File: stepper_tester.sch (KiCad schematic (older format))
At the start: 19 parts, among them J1 Conn_01x08, J2 Conn_01x08, J3 Conn_01x04, J4 Conn_01x03, J5 Conn_01x01, J6 Conn_01x01, J7 Conn_01x01, J8 Conn_01x03, U1 BluePill_STM32F103C

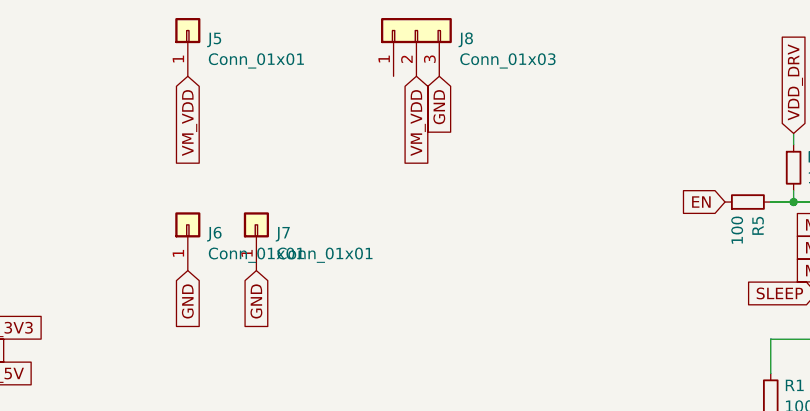
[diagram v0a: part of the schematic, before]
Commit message: Схема
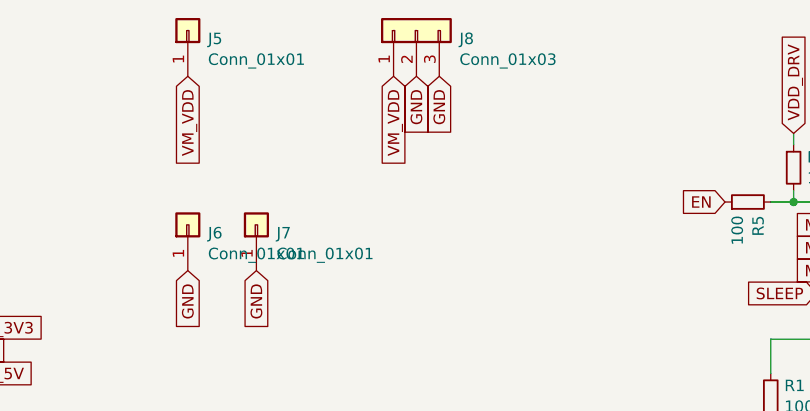
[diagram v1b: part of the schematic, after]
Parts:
- J8: footprint posad:Socket5.5x2.1 -> power:DC55x21THT
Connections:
- net GND: now also J8.2 (Pin_2)
- net VM_VDD: now also J8.1 (Pin_1); no longer J8.2 (Pin_2)
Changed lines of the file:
@@
 F 0 "J8" V 5114 562 50  0000 R CNN
 F 1 "Conn_01x03" V 5023 562 50  0000 R CNN
-F 2 "posad:Socket5.5x2.1" H 5150 750 50  0001 C CNN
+F 2 "power:DC55x21THT" H 5150 750 50  0001 C CNN
 F 3 "~" H 5150 750 50  0001 C CNN
 	1    5150 750
 	0    -1   -1   0
 $EndComp
-Text GLabel 5150 950  3    50   Input ~ 0
+Text GLabel 5050 950  3    50   Input ~ 0
 VM_VDD
 $Comp
@@
 	1    0    0    -1
 $EndComp
+Text GLabel 5150 950  3    50   Input ~ 0
+GND
 $EndSCHEMATC
